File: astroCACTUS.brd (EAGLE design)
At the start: 160 x 100 mm, 21 parts, among them U1 ATTINY85-20P

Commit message: astro boy
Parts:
- moved D18 153.8 mm to (27.8, 18.0), turned to 92.5 degrees
- moved D9 151.3 mm to (32.8, 16.1), turned to 90.7 degrees
- moved D17 142.4 mm to (22.3, 10.7), turned to 92.4 degrees
- moved D8 138.2 mm to (27.9, 12.7), turned to 90.6 degrees
- moved D7 134.9 mm to (22.4, 4.74), turned to 91.8 degrees
- moved D10 129.2 mm to (17.3, 7.87), turned to 91.7 degrees
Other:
- board outline removed
- board text added: "/Users/chrisbuckner/badges/fresh/astro_copper_only.bmp"
- board text added: "/Users/chrisbuckner/badges/fresh/astro_silk_only_no_fire_bitmap.bmp"

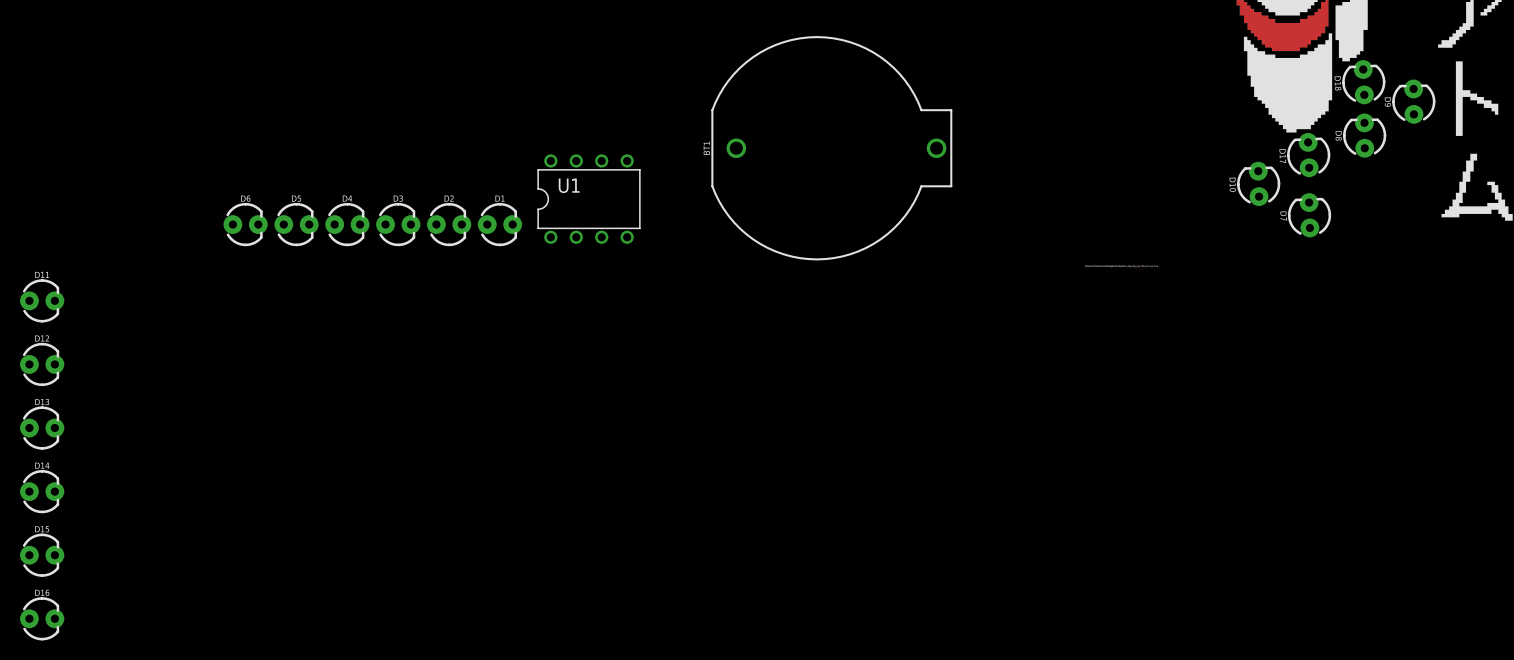
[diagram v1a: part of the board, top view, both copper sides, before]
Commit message: astro boy
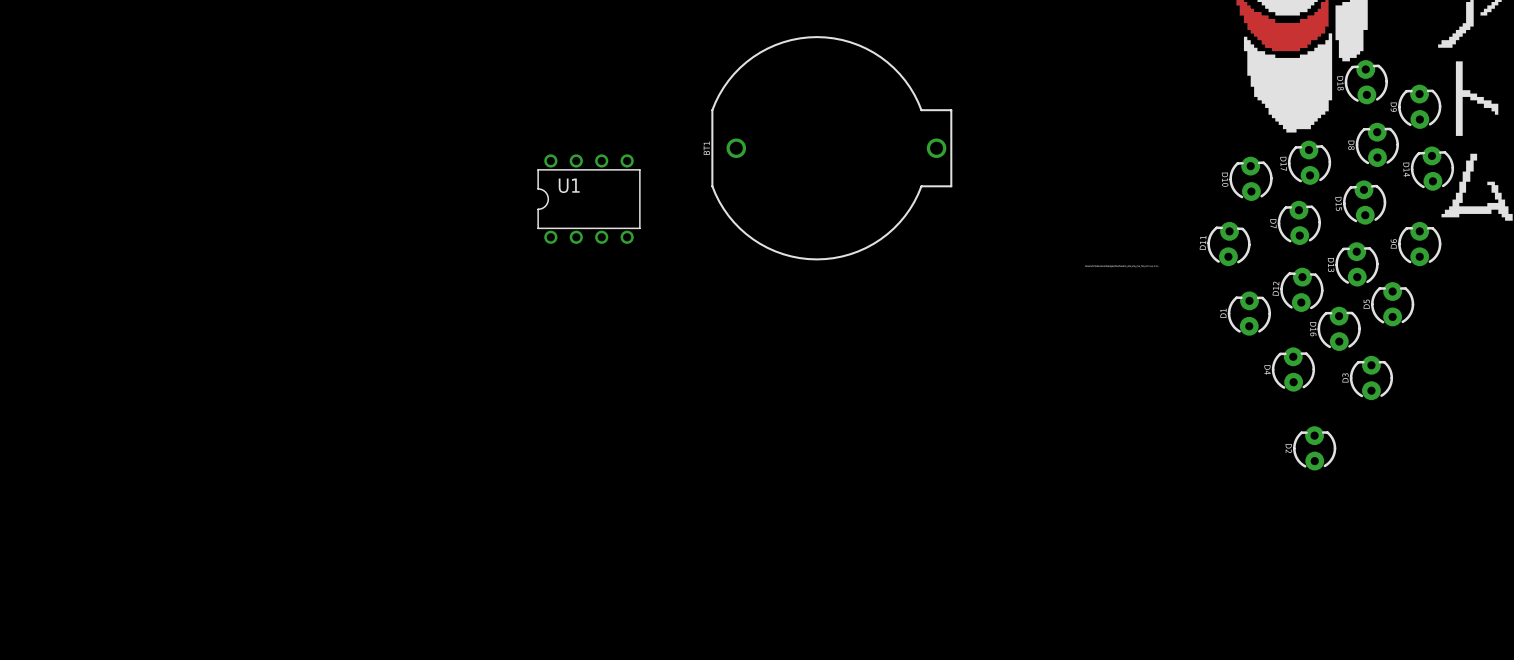
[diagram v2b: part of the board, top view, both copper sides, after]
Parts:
- moved D14 142.5 mm to (34.7, 9.39), turned to 92.1 degrees
- moved D15 136.7 mm to (27.9, 6.01), turned to 93 degrees
- moved D16 132.7 mm to (25.4, -6.61), turned to 90.5 degrees
- moved D13 132.3 mm to (27.2, -0.17), turned to 91.2 degrees
- moved D12 126.0 mm to (21.7, -2.71), turned to 87.5 degrees
- moved D11 118.7 mm to (14.4, 1.86), turned to 87.5 degrees
- moved D6 117.3 mm to (33.4, 1.86), turned to 90 degrees
- moved D5 109.8 mm to (30.7, -4.15), turned to 90 degrees
- moved D3 98.4 mm to (28.6, -11.5), turned to 90 degrees
- moved D4 95.6 mm to (20.8, -10.7), turned to 90.7 degrees
- moved D2 89.3 mm to (22.9, -18.5), turned to 90.4 degrees
- moved D1 75.4 mm to (16.4, -5.08), turned to 89.5 degrees
- moved D8 1.57 mm to (29.2, 11.8)
- moved D7 1.27 mm to (21.4, 3.97)
- moved D10 0.92 mm to (16.6, 8.38)
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
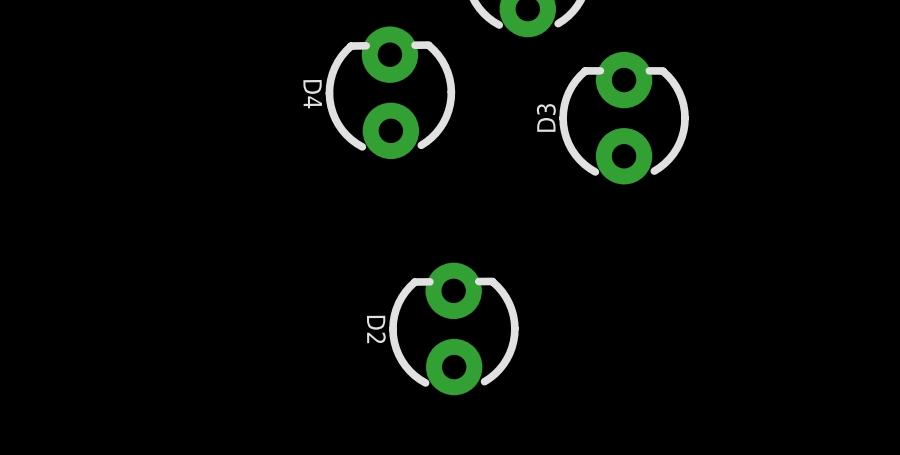
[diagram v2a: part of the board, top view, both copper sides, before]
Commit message: astro boy
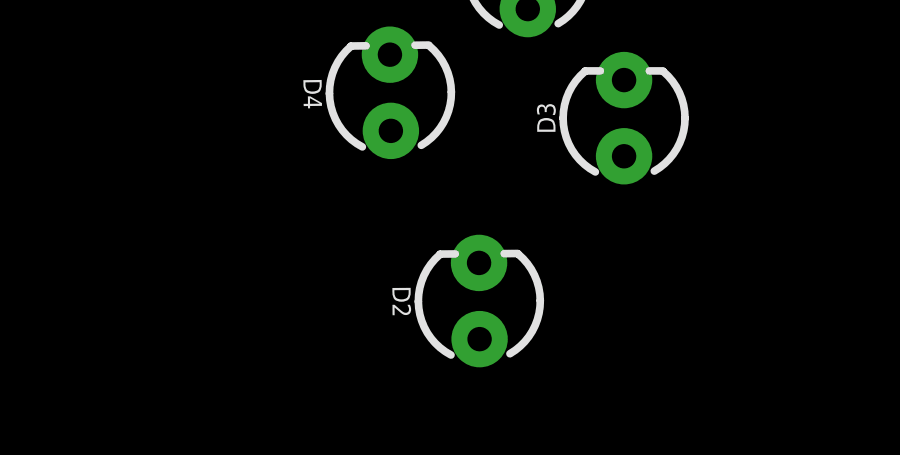
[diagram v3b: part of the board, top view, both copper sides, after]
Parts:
- moved D2 1.26 mm to (23.8, -17.6)
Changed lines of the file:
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@@
 <attribute name="PROD_ID" value="DIO-08794" x="16.41785" y="-5.0791125" size="1.778" layer="27" rot="R89.5" display="off"/>
 </element>
-<element name="D2" library="SparkFun-LED" library_urn="urn:adsk.eagle:library:529" package="LED_3MM" package3d_urn="urn:adsk.eagle:package:39361/1" value="" x="22.936025" y="-18.539765625" rot="R90.4">
-<attribute name="PROD_ID" value="DIO-08794" x="22.936025" y="-18.539765625" size="1.778" layer="27" rot="R90.4" display="off"/>
+<element name="D2" library="SparkFun-LED" library_urn="urn:adsk.eagle:library:529" package="LED_3MM" package3d_urn="urn:adsk.eagle:package:39361/1" value="" x="23.782609375" y="-17.608525" rot="R90.4">
+<attribute name="PROD_ID" value="DIO-08794" x="23.782609375" y="-17.608525" size="1.778" layer="27" rot="R90.4" display="off"/>
 </element>
 <element name="D3" library="SparkFun-LED" library_urn="urn:adsk.eagle:library:529" package="LED_3MM" package3d_urn="urn:adsk.eagle:package:39361/1" value="" x="28.607609375" y="-11.513140625" rot="R90">
@@
 <wire x1="20.8340625" y1="-11.936453125" x2="30.72305625" y2="-5.41786875" width="0" layer="19" extent="1-1"/>
 <wire x1="28.607609375" y1="-12.783140625" x2="20.8340625" y2="-11.936453125" width="0" layer="19" extent="1-1"/>
-<wire x1="22.944890625" y1="-19.809734375" x2="28.607609375" y2="-12.783140625" width="0" layer="19" extent="1-1"/>
-<wire x1="16.406765625" y1="-6.3490625" x2="22.944890625" y2="-19.809734375" width="0" layer="19" extent="1-1"/>
+<wire x1="23.791475" y1="-18.87849375" x2="28.607609375" y2="-12.783140625" width="0" layer="19" extent="1-1"/>
+<wire x1="16.406765625" y1="-6.3490625" x2="23.791475" y2="-18.87849375" width="0" layer="19" extent="1-1"/>
 <wire x1="-53.34" y1="10.16" x2="16.406765625" y2="-6.3490625" width="0" layer="19" extent="1-1"/>
 <wire x1="-44.45" y1="48.26" x2="-53.34" y2="10.16" width="0" layer="19" extent="1-1"/>
@@
 <wire x1="20.803034375" y1="-9.39664375" x2="30.72305625" y2="-2.87786875" width="0" layer="19" extent="1-1"/>
 <wire x1="28.607609375" y1="-10.243140625" x2="20.803034375" y2="-9.39664375" width="0" layer="19" extent="1-1"/>
-<wire x1="22.92715625" y1="-17.26979375" x2="28.607609375" y2="-10.243140625" width="0" layer="19" extent="1-1"/>
-<wire x1="16.42893125" y1="-3.809159375" x2="22.92715625" y2="-17.26979375" width="0" layer="19" extent="1-1"/>
+<wire x1="23.773740625" y1="-16.338553125" x2="28.607609375" y2="-10.243140625" width="0" layer="19" extent="1-1"/>
+<wire x1="16.42893125" y1="-3.809159375" x2="23.773740625" y2="-16.338553125" width="0" layer="19" extent="1-1"/>
 <wire x1="-50.8" y1="2.54" x2="16.42893125" y2="-3.809159375" width="0" layer="19" extent="1-1"/>
 </signal>

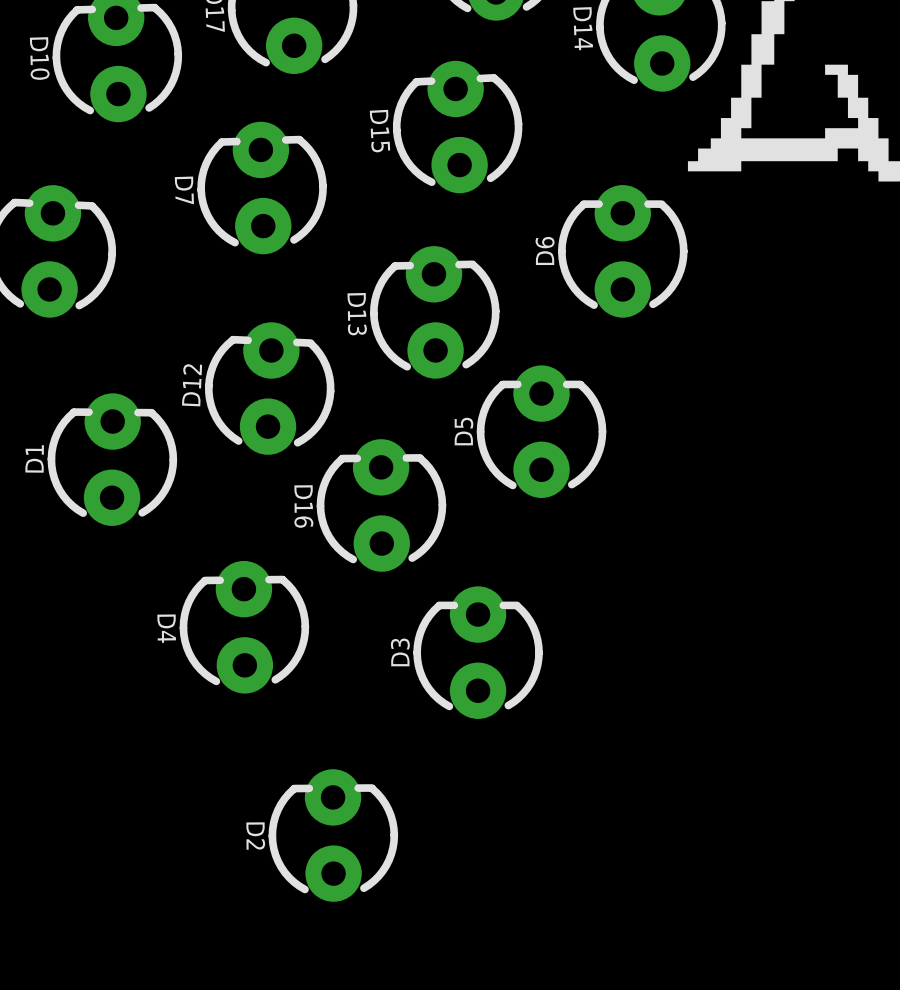
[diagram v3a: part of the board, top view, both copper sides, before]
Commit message: astro boy
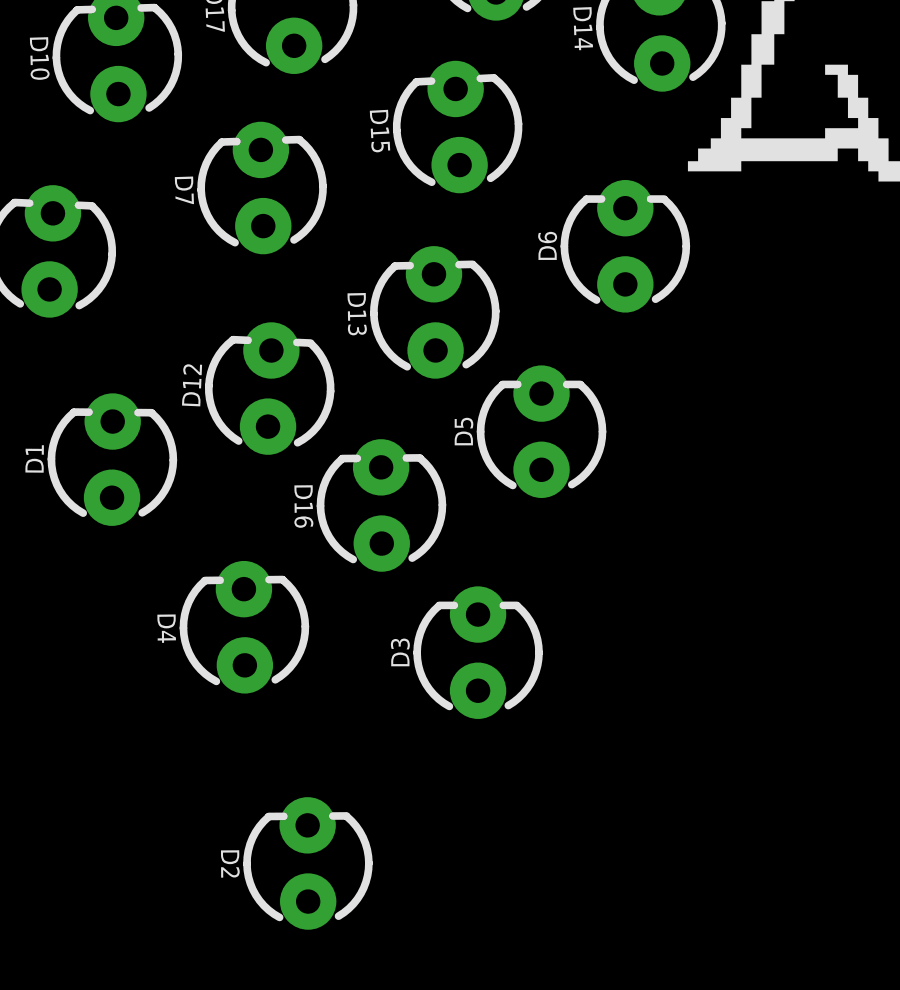
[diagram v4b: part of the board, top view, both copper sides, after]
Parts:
- moved D2 1.26 mm to (22.9, -18.5)
- moved D6 0.19 mm to (33.5, 2.03)
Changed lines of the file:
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@@
 <attribute name="PROD_ID" value="DIO-08794" x="16.41785" y="-5.0791125" size="1.778" layer="27" rot="R89.5" display="off"/>
 </element>
-<element name="D2" library="SparkFun-LED" library_urn="urn:adsk.eagle:library:529" package="LED_3MM" package3d_urn="urn:adsk.eagle:package:39361/1" value="" x="23.782609375" y="-17.608525" rot="R90.4">
-<attribute name="PROD_ID" value="DIO-08794" x="23.782609375" y="-17.608525" size="1.778" layer="27" rot="R90.4" display="off"/>
+<element name="D2" library="SparkFun-LED" library_urn="urn:adsk.eagle:library:529" package="LED_3MM" package3d_urn="urn:adsk.eagle:package:39361/1" value="" x="22.936025" y="-18.539765625" rot="R90.4">
+<attribute name="PROD_ID" value="DIO-08794" x="22.936025" y="-18.539765625" size="1.778" layer="27" rot="R90.4" display="off"/>
 </element>
 <element name="D3" library="SparkFun-LED" library_urn="urn:adsk.eagle:library:529" package="LED_3MM" package3d_urn="urn:adsk.eagle:package:39361/1" value="" x="28.607609375" y="-11.513140625" rot="R90">
@@
 <attribute name="PROD_ID" value="DIO-08794" x="30.72305625" y="-4.14786875" size="1.778" layer="27" rot="R90" display="off"/>
 </element>
-<element name="D6" library="SparkFun-LED" library_urn="urn:adsk.eagle:library:529" package="LED_3MM" package3d_urn="urn:adsk.eagle:package:39361/1" value="" x="33.431609375" y="1.8628625" rot="R90">
-<attribute name="PROD_ID" value="DIO-08794" x="33.431609375" y="1.8628625" size="1.778" layer="27" rot="R90" display="off"/>
+<element name="D6" library="SparkFun-LED" library_urn="urn:adsk.eagle:library:529" package="LED_3MM" package3d_urn="urn:adsk.eagle:package:39361/1" value="" x="33.51626875" y="2.03218125" rot="R90">
+<attribute name="PROD_ID" value="DIO-08794" x="33.51626875" y="2.03218125" size="1.778" layer="27" rot="R90" display="off"/>
 </element>
 <element name="D11" library="SparkFun-LED" library_urn="urn:adsk.eagle:library:529" package="LED_3MM" package3d_urn="urn:adsk.eagle:package:39361/1" value="" x="14.3814875" y="1.862096875" rot="R87.5">
@@
 <wire x1="21.448003125" y1="2.705375" x2="22.477190625" y2="8.715321875" width="0" layer="19" extent="1-1"/>
 <wire x1="14.326090625" y1="0.59330625" x2="21.448003125" y2="2.705375" width="0" layer="19" extent="1-1"/>
-<wire x1="33.431609375" y1="0.5928625" x2="14.326090625" y2="0.59330625" width="0" layer="19" extent="1-1"/>
-<wire x1="30.72305625" y1="-5.41786875" x2="33.431609375" y2="0.5928625" width="0" layer="19" extent="1-1"/>
+<wire x1="33.51626875" y1="0.76218125" x2="14.326090625" y2="0.59330625" width="0" layer="19" extent="1-1"/>
+<wire x1="30.72305625" y1="-5.41786875" x2="33.51626875" y2="0.76218125" width="0" layer="19" extent="1-1"/>
 <wire x1="20.8340625" y1="-11.936453125" x2="30.72305625" y2="-5.41786875" width="0" layer="19" extent="1-1"/>
 <wire x1="28.607609375" y1="-12.783140625" x2="20.8340625" y2="-11.936453125" width="0" layer="19" extent="1-1"/>
-<wire x1="23.791475" y1="-18.87849375" x2="28.607609375" y2="-12.783140625" width="0" layer="19" extent="1-1"/>
-<wire x1="16.406765625" y1="-6.3490625" x2="23.791475" y2="-18.87849375" width="0" layer="19" extent="1-1"/>
+<wire x1="22.944890625" y1="-19.809734375" x2="28.607609375" y2="-12.783140625" width="0" layer="19" extent="1-1"/>
+<wire x1="16.406765625" y1="-6.3490625" x2="22.944890625" y2="-19.809734375" width="0" layer="19" extent="1-1"/>
 <wire x1="-53.34" y1="10.16" x2="16.406765625" y2="-6.3490625" width="0" layer="19" extent="1-1"/>
 <wire x1="-44.45" y1="48.26" x2="-53.34" y2="10.16" width="0" layer="19" extent="1-1"/>
@@
 <contactref element="D5" pad="K"/>
 <contactref element="D6" pad="K"/>
-<wire x1="30.72305625" y1="-2.87786875" x2="33.431609375" y2="3.1328625" width="0" layer="19" extent="1-1"/>
+<wire x1="30.72305625" y1="-2.87786875" x2="33.51626875" y2="3.30218125" width="0" layer="19" extent="1-1"/>
 <wire x1="20.803034375" y1="-9.39664375" x2="30.72305625" y2="-2.87786875" width="0" layer="19" extent="1-1"/>
 <wire x1="28.607609375" y1="-10.243140625" x2="20.803034375" y2="-9.39664375" width="0" layer="19" extent="1-1"/>
-<wire x1="23.773740625" y1="-16.338553125" x2="28.607609375" y2="-10.243140625" width="0" layer="19" extent="1-1"/>
-<wire x1="16.42893125" y1="-3.809159375" x2="23.773740625" y2="-16.338553125" width="0" layer="19" extent="1-1"/>
+<wire x1="22.92715625" y1="-17.26979375" x2="28.607609375" y2="-10.243140625" width="0" layer="19" extent="1-1"/>
+<wire x1="16.42893125" y1="-3.809159375" x2="22.92715625" y2="-17.26979375" width="0" layer="19" extent="1-1"/>
 <wire x1="-50.8" y1="2.54" x2="16.42893125" y2="-3.809159375" width="0" layer="19" extent="1-1"/>
 </signal>
